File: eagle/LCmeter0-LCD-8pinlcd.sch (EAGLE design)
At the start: 26 parts, among them IC1 PIC16F876A-X/SP, K2 DS2Y, Q1 20MHz, Q2 BC548, SW1 SPST, X2 C-GRID-02-70543

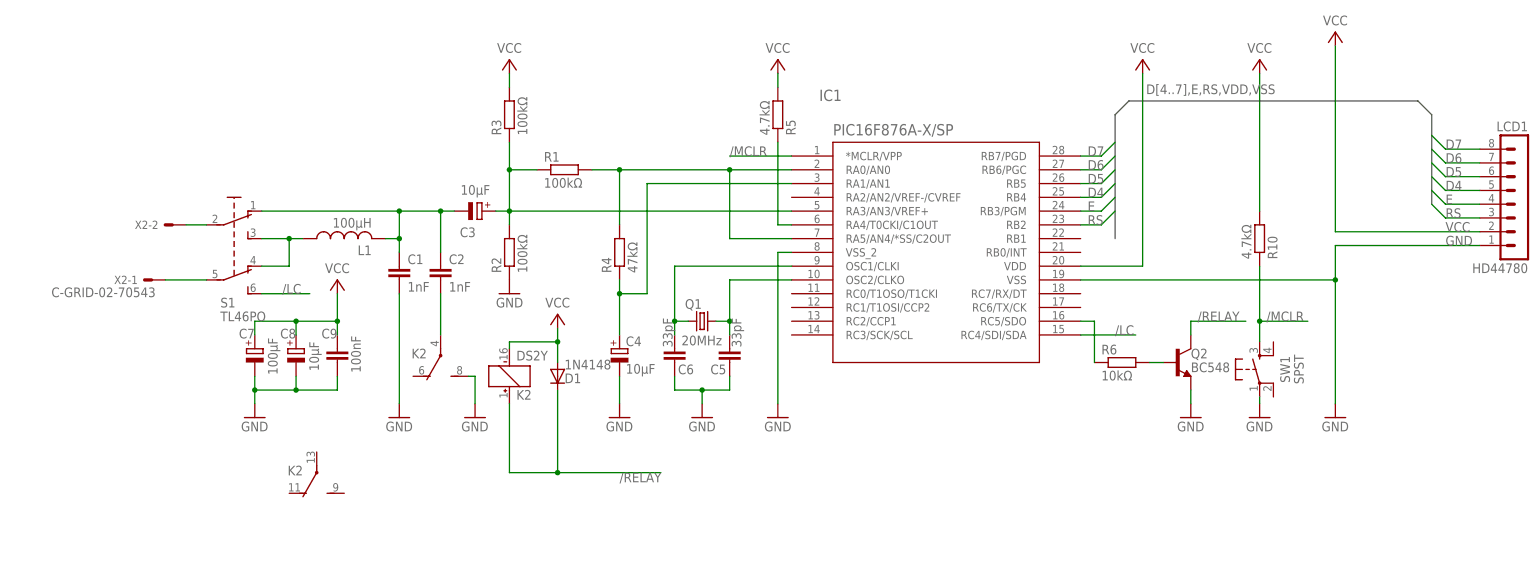
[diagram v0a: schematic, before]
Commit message: ...
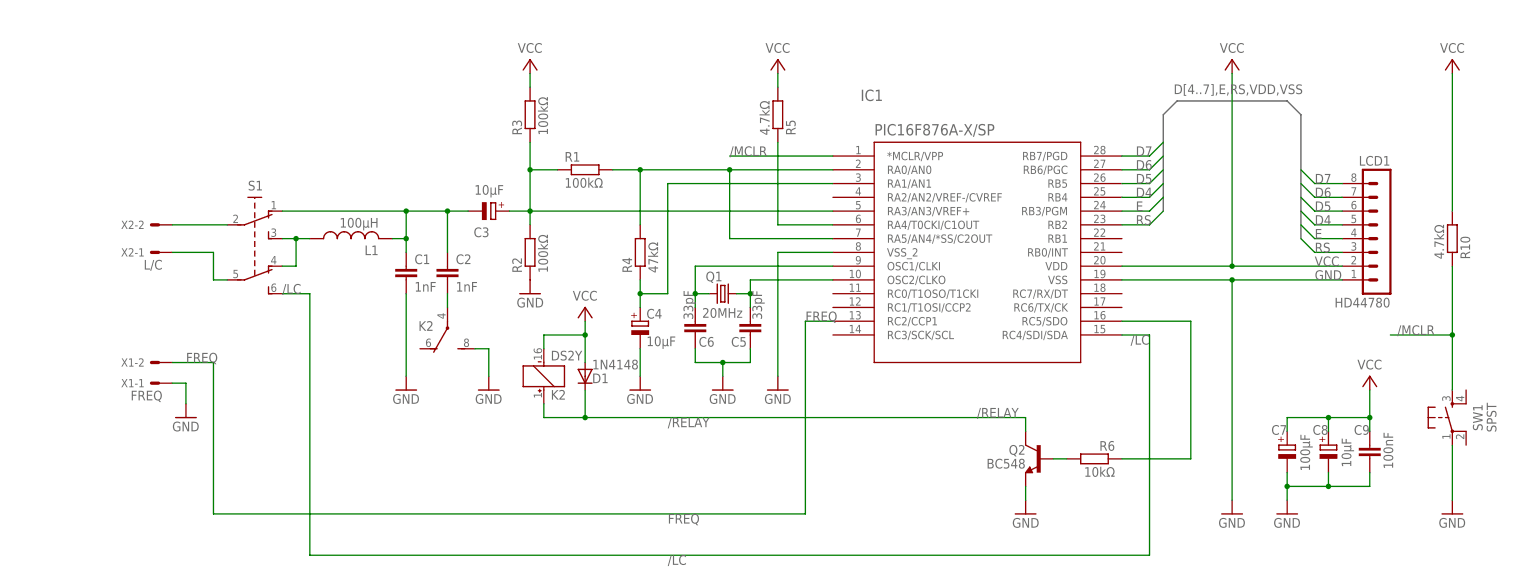
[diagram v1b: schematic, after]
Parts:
- added X1: FREQ, con-molex:C-GRID-02-70543
- R5: device resistor:R-EU_0204/2V -> resistor:R-EU_0207/10
- X2: value C-GRID-02-70543 -> L/C
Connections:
- new net FREQ: IC1.RC2/CCP1, X1-2.S
- net GND: now also X1-1.S
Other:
- moved on the sheet: C1, C2, C3, C4, C5, C6, C7, C8, C9, D1, IC1, K2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
